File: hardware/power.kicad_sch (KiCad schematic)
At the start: 4 parts, among them U2 TPS54360DDA, U3 AP7361C-33E, U4 R-78HB5.0-0.5

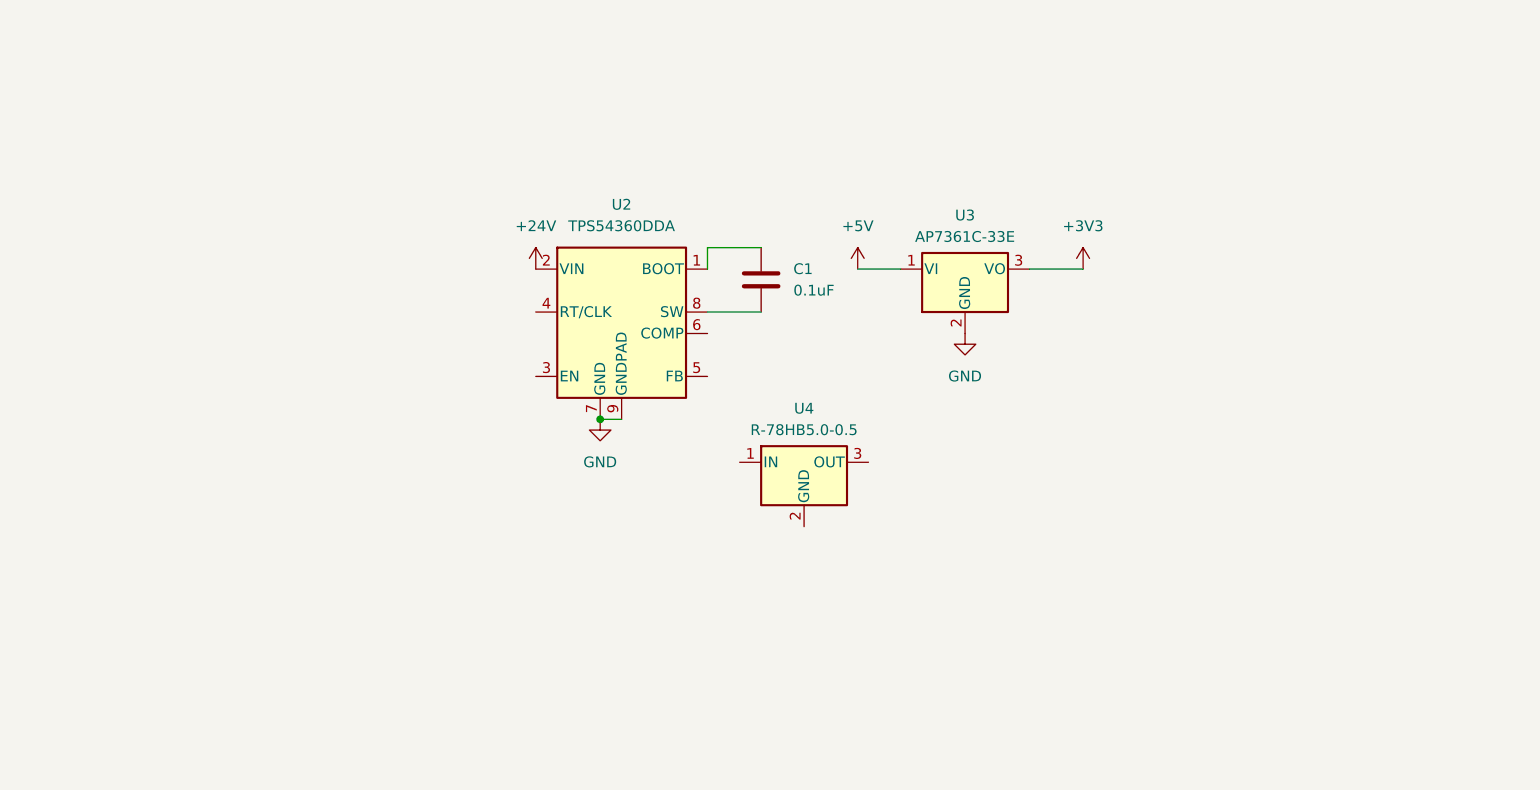
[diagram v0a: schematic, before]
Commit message: make the schematics
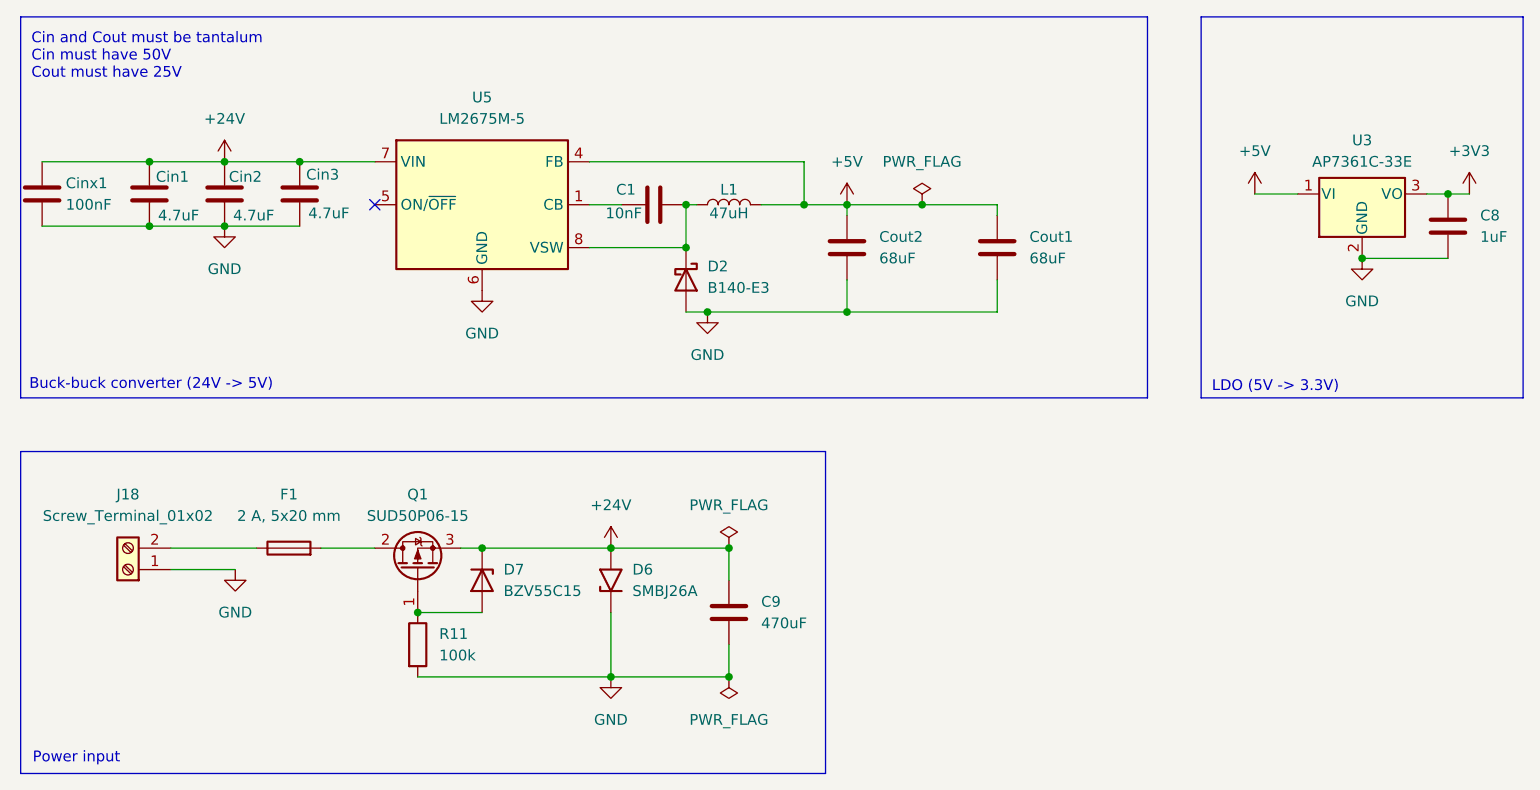
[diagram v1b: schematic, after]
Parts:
- removed U2: TPS54360DDA, Package_SO:TI_SO-PowerPAD-8_ThermalVias, symbol Regulator_Switching:TPS54360DDA
- removed U4: R-78HB5.0-0.5, Converter_DCDC:Converter_DCDC_RECOM_R-78HB-0.5_THT, symbol Converter_DCDC:R-78HB5.0-0.5
- added C8: 1uF, symbol Device:C
- added C9: 470uF, symbol Device:C
- added Cin1, Cin2, Cin3: 4.7uF, symbol Device:C
- added Cinx1: 100nF, symbol Device:C
- added Cout1, Cout2: 68uF, symbol Device:C
- added D2: B140-E3, Diode_SMD:D_SMA, symbol Diode:B140-E3
- added D6: SMBJ26A, Diode_SMD:D_SMB, symbol Diode:SM6T33A
- added D7: BZV55C15, Diode_SMD:D_MiniMELF, symbol Diode:BZV55C15
- added F1: 2 A, 5x20 mm, Fuse:Fuseholder_Cylinder-5x20mm_Stelvio-Kontek_PTF78_Horizontal_Open, symbol Device:Fuse
- added J18: Screw_Terminal_01x02, symbol Connector:Screw_Terminal_01x02
- added L1: 47uH, symbol Device:L
- added Q1: SUD50P06-15, Package_TO_SOT_SMD:TO-252-2, symbol Transistor_FET:SUD50P06-15
- added R11: 100k, symbol Device:R
- added U5: LM2675M-5, Package_SO:SOIC-8_3.9x4.9mm_P1.27mm, symbol Regulator_Switching:LM2675M-5
- C1: value 0.1uF -> 10nF
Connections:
- net +24V: now also C9.2, Cin1.2, Cin2.2, Cin3.2, Cinx1.2, D6.2 (A2), D7.1 (K), Q1.3 (S), U5.7 (VIN)
- net +3V3: now also C8.1
- net +5V: now also Cout1.2, Cout2.2, L1.2, U5.4 (FB)
- net GND: now also C8.2, C9.1, Cin1.1, Cin2.1, Cin3.1, Cinx1.1, Cout1.1, Cout2.1, D2.2 (A), D6.1 (A1), J18.1 (Pin_1), R11.2, U5.6 (GND)
- net at C1.1: now also U5.1 (CB)
- net at C1.2: now also D2.1 (K), L1.1, U5.8 (VSW)
- new net: D7.2 (A), Q1.1 (G), R11.1
- new net: F1.2, Q1.2 (D)
- new net: F1.1, J18.2 (Pin_2)
- no-connect marks 0 -> 1
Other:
- note added: "Buck-buck converter (24V -> 5V)"
- note added: "Cin and Cout must be tantalum Cin must have 50V Cout must have 25V"
- note added: "LDO (5V -> 3.3V)"
- note added: "Power input"
- moved on the sheet: U3
